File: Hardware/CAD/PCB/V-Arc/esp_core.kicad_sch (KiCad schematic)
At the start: 23 parts, among them J4 AudioJack2, J5 AudioJack3, J6 AudioJack2, SW10 SW_Push, SW11 SW_Push, U7 XIAO-ESP32-S3-SMD, U8 ER_OLEDM0.91_1x-I2C, U9 TL072

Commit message: Assigned Footprints
-Swapped input jack to a switched one
-Assigned footprints for all items
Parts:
- C25, C26, C31, C32: footprint (none) -> Capacitor_SMD:C_0805_2012Metric
- C27, C28, C29, C30: footprint (none) -> Capacitor_SMD:CP_Elec_6.3x5.4
- J4, J6: footprint (none) -> Connector_Audio:Jack_3.5mm_CUI_SJ1-3513N_Horizontal
- J5: footprint (none) -> Connector_Audio:Jack_3.5mm_CUI_SJ1-3523N_Horizontal
- R15, R16, R17, R18, R19, R20: footprint (none) -> Resistor_SMD:R_0805_2012Metric
- RV6: footprint (none) -> Potentiometer_THT:Potentiometer_Bourns_PTV09A-1_Single_Vertical
- SW10, SW11: footprint (none) -> Button_Switch_THT:SW_PUSH-12mm_Wuerth-430476085716
- U9: footprint (none) -> Package_SO:SOIC-8_3.9x4.9mm_P1.27mm
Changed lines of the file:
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@@
 			)
 		)
-		(property "Footprint" ""
+		(property "Footprint" "Package_SO:SOIC-8_3.9x4.9mm_P1.27mm"
 			(at 123.19 116.84 0)
 			(hide yes)
@@
 			)
 		)
-		(property "Footprint" ""
+		(property "Footprint" "Capacitor_SMD:C_0805_2012Metric"
 			(at 134.62 147.32 0)
 			(hide yes)
@@
 			)
 		)
-		(property "Footprint" ""
+		(property "Footprint" "Capacitor_SMD:C_0805_2012Metric"
 			(at 106.68 147.32 0)
 			(hide yes)
@@
 			)
 		)
-		(property "Footprint" ""
+		(property "Footprint" "Resistor_SMD:R_0805_2012Metric"
 			(at 87.63 113.03 0)
 			(hide yes)
@@
 			)
 		)
-		(property "Footprint" ""
+		(property "Footprint" "Potentiometer_THT:Potentiometer_Bourns_PTV09A-1_Single_Vertical"
 			(at 102.235 127 0)
 			(hide yes)
@@
 			)
 		)
-		(property "Footprint" ""
+		(property "Footprint" "Package_SO:SOIC-8_3.9x4.9mm_P1.27mm"
 			(at 123.19 142.24 0)
 			(hide yes)
@@
 			)
 		)
-		(property "Footprint" ""
+		(property "Footprint" "Button_Switch_THT:SW_PUSH-12mm_Wuerth-430476085716"
 			(at 119.38 50.8 0)
 			(hide yes)
@@
 			)
 		)
-		(property "Footprint" ""
+		(property "Footprint" "Resistor_SMD:R_0805_2012Metric"
 			(at 87.63 135.89 0)
 			(hide yes)
@@
 			)
 		)
-		(property "Footprint" ""
+		(property "Footprint" "Resistor_SMD:R_0805_2012Metric"
 			(at 137.16 116.84 0)
 			(hide yes)
@@
 			)
 		)
-		(property "Footprint" ""
+		(property "Footprint" "Connector_Audio:Jack_3.5mm_CUI_SJ1-3523N_Horizontal"
 			(at 215.9 124.46 0)
 			(hide yes)
@@
 			)
 		)
-		(property "Footprint" ""
+		(property "Footprint" "Button_Switch_THT:SW_PUSH-12mm_Wuerth-430476085716"
 			(at 124.46 50.8 0)
 			(hide yes)
@@
 			)
 		)
-		(property "Footprint" ""
+		(property "Footprint" "Connector_Audio:Jack_3.5mm_CUI_SJ1-3513N_Horizontal"
 			(at 215.9 114.3 0)
 			(hide yes)
@@
 			)
 		)
-		(property "Footprint" ""
+		(property "Footprint" "Resistor_SMD:R_0805_2012Metric"
 			(at 152.4 114.3 0)
 			(hide yes)
@@
 			)
 		)
-		(property "Footprint" ""
+		(property "Footprint" "Resistor_SMD:R_0805_2012Metric"
 			(at 152.4 132.08 0)
 			(hide yes)
@@
 			)
 		)
-		(property "Footprint" ""
+		(property "Footprint" "Capacitor_SMD:CP_Elec_6.3x5.4"
 			(at 146.05 129.54 0)
 			(hide yes)
@@
 			)
 		)
-		(property "Footprint" ""
+		(property "Footprint" "Package_SO:SOIC-8_3.9x4.9mm_P1.27mm"
 			(at 123.19 129.54 0)
 			(hide yes)
@@
 			)
 		)
-		(property "Footprint" ""
+		(property "Footprint" "Connector_Audio:Jack_3.5mm_CUI_SJ1-3513N_Horizontal"
 			(at 215.9 106.68 0)
 			(hide yes)
@@
 			)
 		)
-		(property "Footprint" ""
+		(property "Footprint" "Capacitor_SMD:CP_Elec_6.3x5.4"
 			(at 80.01 118.11 0)
 			(hide yes)
@@
 			)
 		)
-		(property "Footprint" ""
+		(property "Footprint" "Capacitor_SMD:CP_Elec_6.3x5.4"
 			(at 80.01 130.81 0)
 			(hide yes)
@@
 			)
 		)
-		(property "Footprint" ""
+		(property "Footprint" "Capacitor_SMD:C_0805_2012Metric"
 			(at 121.92 62.23 0)
 			(hide yes)
@@
 			)
 		)
-		(property "Footprint" ""
+		(property "Footprint" "Capacitor_SMD:CP_Elec_6.3x5.4"
 			(at 146.05 116.84 0)
 			(hide yes)
@@
 			)
 		)
-		(property "Footprint" ""
+		(property "Footprint" "Capacitor_SMD:C_0805_2012Metric"
 			(at 111.76 63.5 0)
 			(hide yes)
@@
 			)
 		)
-		(property "Footprint" ""
+		(property "Footprint" "Resistor_SMD:R_0805_2012Metric"
 			(at 137.16 129.54 0)
 			(hide yes)

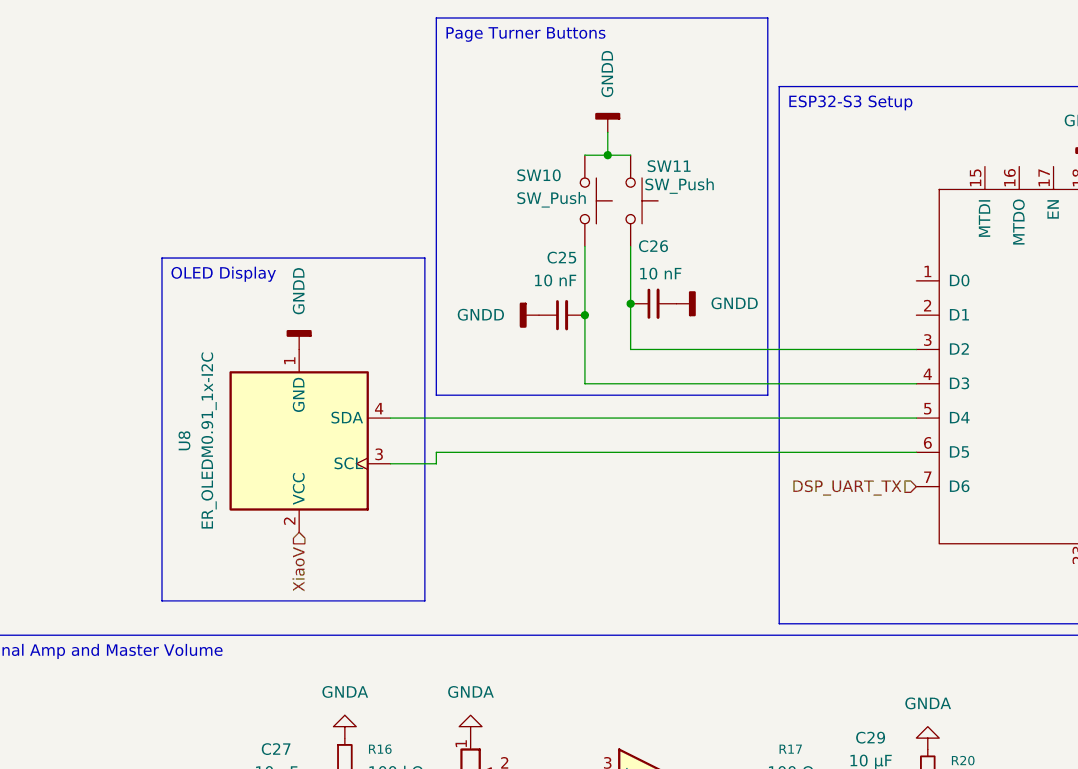
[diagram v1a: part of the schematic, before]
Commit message: Finished PCB Layout
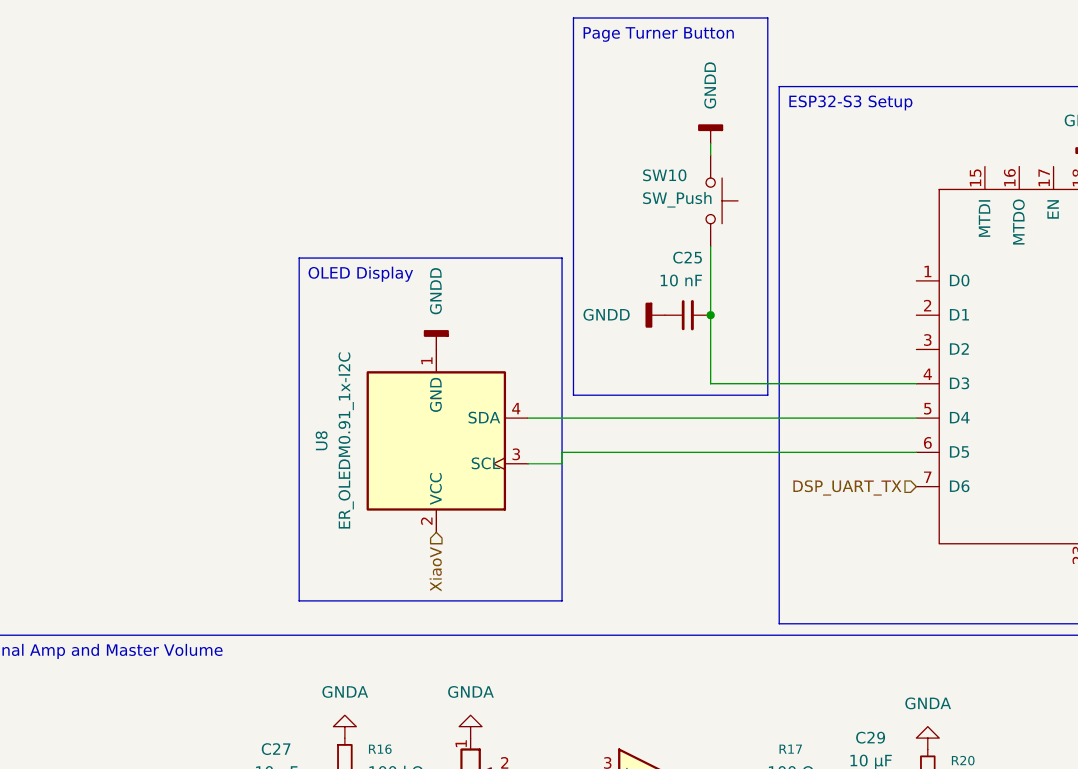
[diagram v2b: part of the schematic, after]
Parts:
- removed C26: 10 nF, Capacitor_SMD:C_0805_2012Metric, symbol Device:C_Small
- removed SW11: SW_Push, Button_Switch_THT:SW_PUSH-12mm_Wuerth-430476085716, symbol Switch:SW_Push
- RV6: footprint Potentiometer_THT:Potentiometer_Bourns_PTV09A-1_Single_Vertical -> Potentiometer_THT:Potentiometer_Alpha_RD902F-40-00D_Dual_Vertical
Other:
- moved on the sheet: C25, SW10, U8
